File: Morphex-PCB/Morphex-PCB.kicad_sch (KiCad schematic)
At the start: 37 parts, among them IC1 TXB0108PWR, IC2 NC7WZ241K8X, J1 Main Terminal, U1 DEV-16771, U2 NRF24, U3 BNO055

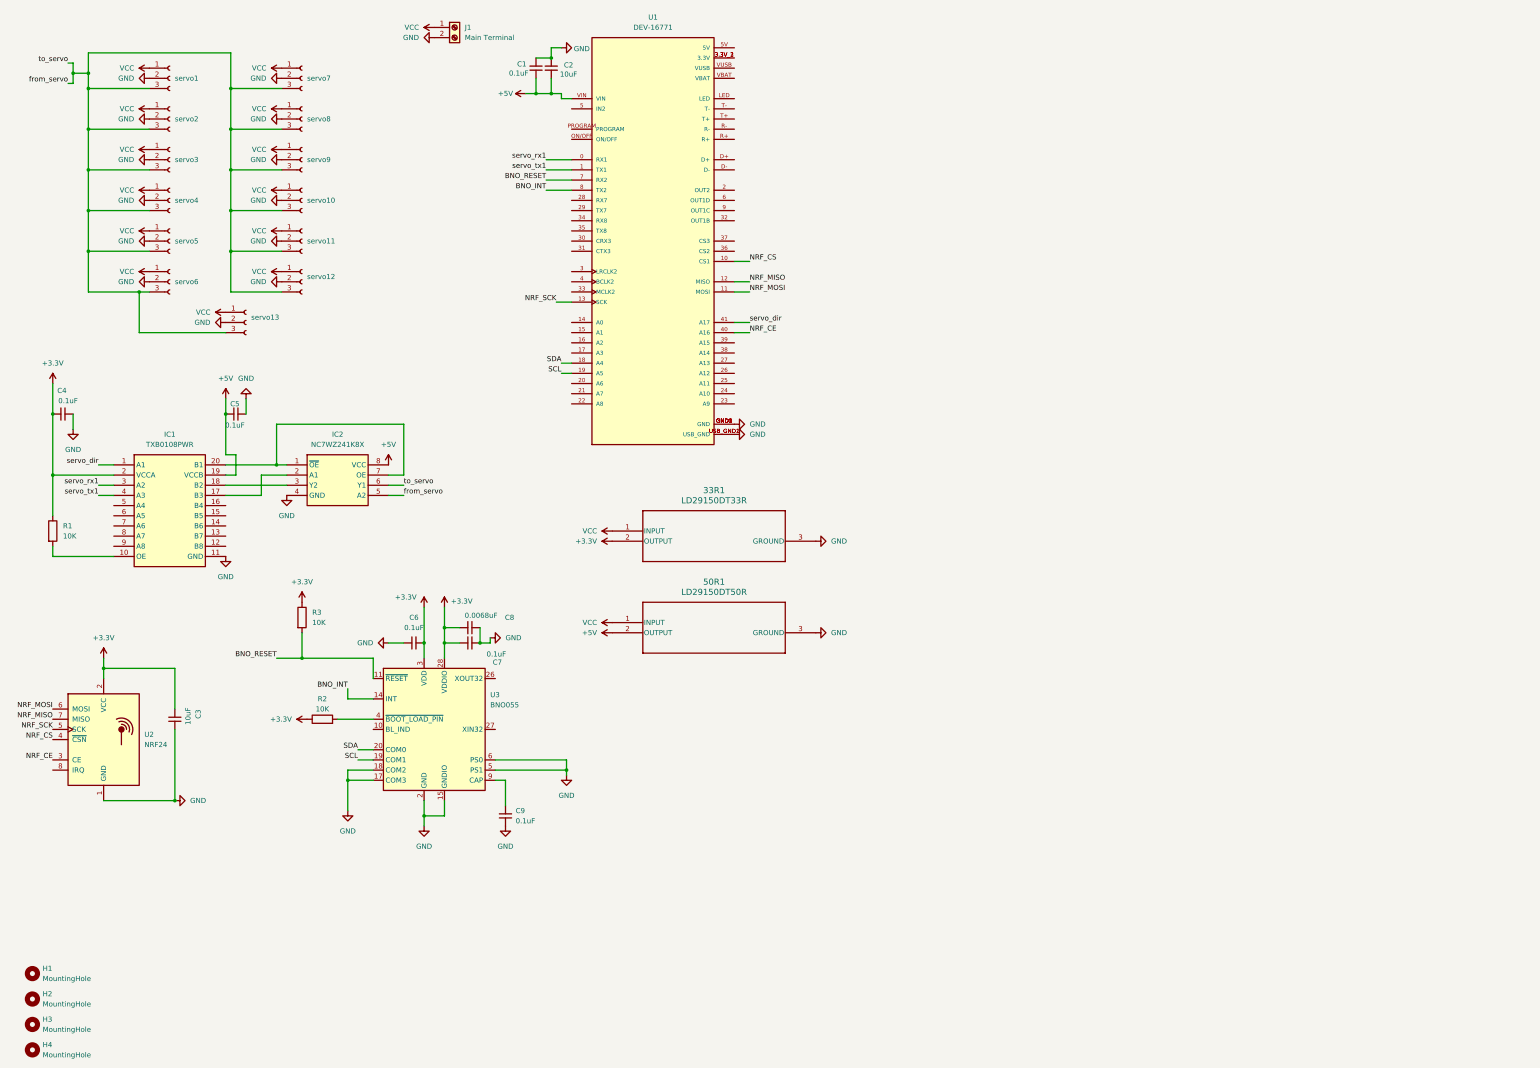
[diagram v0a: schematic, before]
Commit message: update pcb
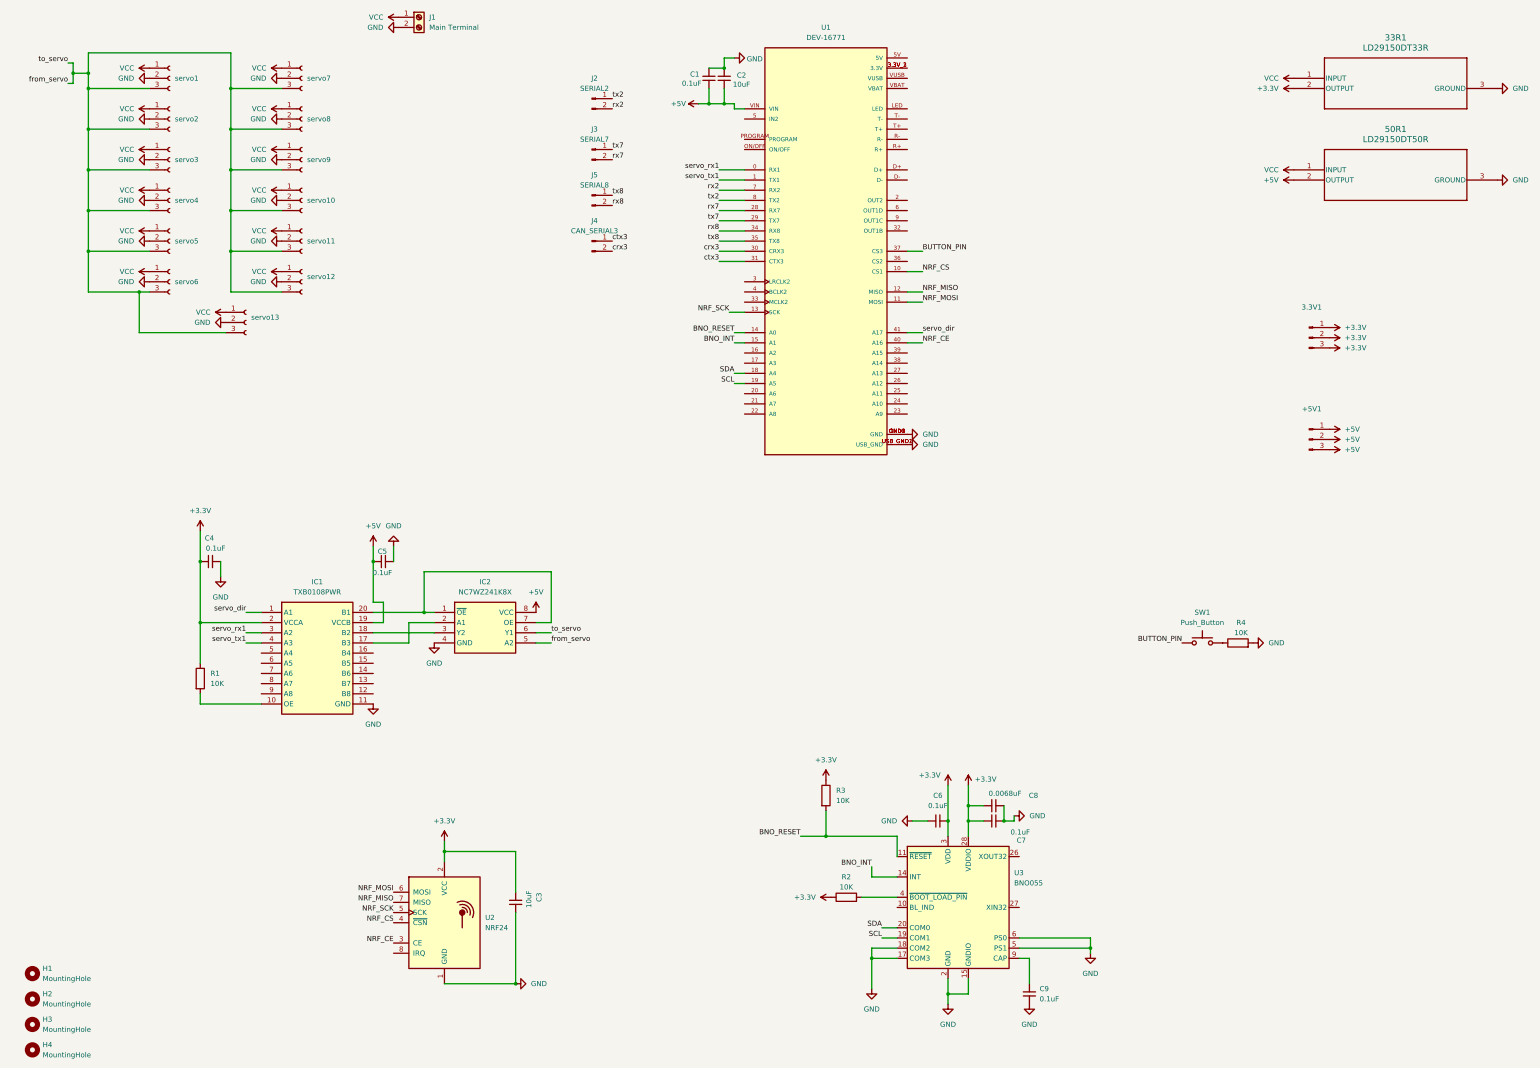
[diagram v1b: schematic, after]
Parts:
- added +5V1, 3.3V1: Conn_01x03_Pin, Connector_PinHeader_2.54mm:PinHeader_1x03_P2.54mm_Vertical, symbol Connector:Conn_01x03_Pin
- added J2: SERIAL2, Connector_PinHeader_2.54mm:PinHeader_1x02_P2.54mm_Vertical, symbol Connector:Conn_01x02_Pin
- added J3: SERIAL7, Connector_PinHeader_2.54mm:PinHeader_1x02_P2.54mm_Vertical, symbol Connector:Conn_01x02_Pin
- added J4: CAN_SERIAL3, Connector_PinHeader_2.54mm:PinHeader_1x02_P2.54mm_Vertical, symbol Connector:Conn_01x02_Pin
- added J5: SERIAL8, Connector_PinHeader_2.54mm:PinHeader_1x02_P2.54mm_Vertical, symbol Connector:Conn_01x02_Pin
- added R4: 10K, Resistor_SMD:R_0603_1608Metric_Pad0.98x0.95mm_HandSolder, symbol Device:R
- added SW1: Push_Button, Button_Switch_THT:SW_PUSH_6mm, symbol Switch:SW_Push
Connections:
- net +3.3V: now also 3.3V1.1 (Pin_1), 3.3V1.2 (Pin_2), 3.3V1.3 (Pin_3)
- net +5V: now also +5V1.1 (Pin_1), +5V1.2 (Pin_2), +5V1.3 (Pin_3)
- net BNO_INT: now also U1.15 (A1); no longer U1.8 (TX2)
- net BNO_RESET: now also U1.14 (A0); no longer U1.7 (RX2)
- net GND: now also R4.2
- net rx7: now reaches U1.28 (RX7)
- net rx7: now also J3.2 (Pin_2)
- net tx7: now reaches U1.29 (TX7)
- net tx7: now also J3.1 (Pin_1)
- net crx3: now reaches U1.30 (CRX3)
- net crx3: now also J4.2 (Pin_2)
- net ctx3: now reaches U1.31 (CTX3)
- net ctx3: now also J4.1 (Pin_1)
- net rx8: now reaches U1.34 (RX8)
- net rx8: now also J5.2 (Pin_2)
- net tx8: now reaches U1.35 (TX8)
- net tx8: now also J5.1 (Pin_1)
- net BUTTON_PIN: now reaches U1.37 (CS3)
- net BUTTON_PIN: now also SW1.1
- new net: R4.1, SW1.2
- new net rx2: J2.2 (Pin_2), U1.7 (RX2)
- new net tx2: J2.1 (Pin_1), U1.8 (TX2)
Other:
- moved on the sheet: 33R1, 50R1, C1, C2, C3, C4, C5, C6, C7, C8, C9, IC1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
